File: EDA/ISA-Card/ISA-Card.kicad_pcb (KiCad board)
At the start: 2 copper layers, 138.4 x 98.4 mm, 161 parts, among them U7101 74HCT245, U7102 74HCT244, U7104 74HCT138, U7105 74HCT138, U7106 74LS08, U7107 74LS32, U7108 74LS32, U7109 74HC368, U7110 74HC04, U7111 74HC125, U7112 74HC74, U7113 74HC74, U7114 74HC4024, U7115 74HC4024, U7116 74HC595, U7117 74HC595, U7118 74HC595, U7119 8251, U7120 26LS31, U7121 26LS32, X2 Conn_02x04_Counter_Clockwise, X3 DB15_Female, X5 Conn_02x08_Counter_Clockwise

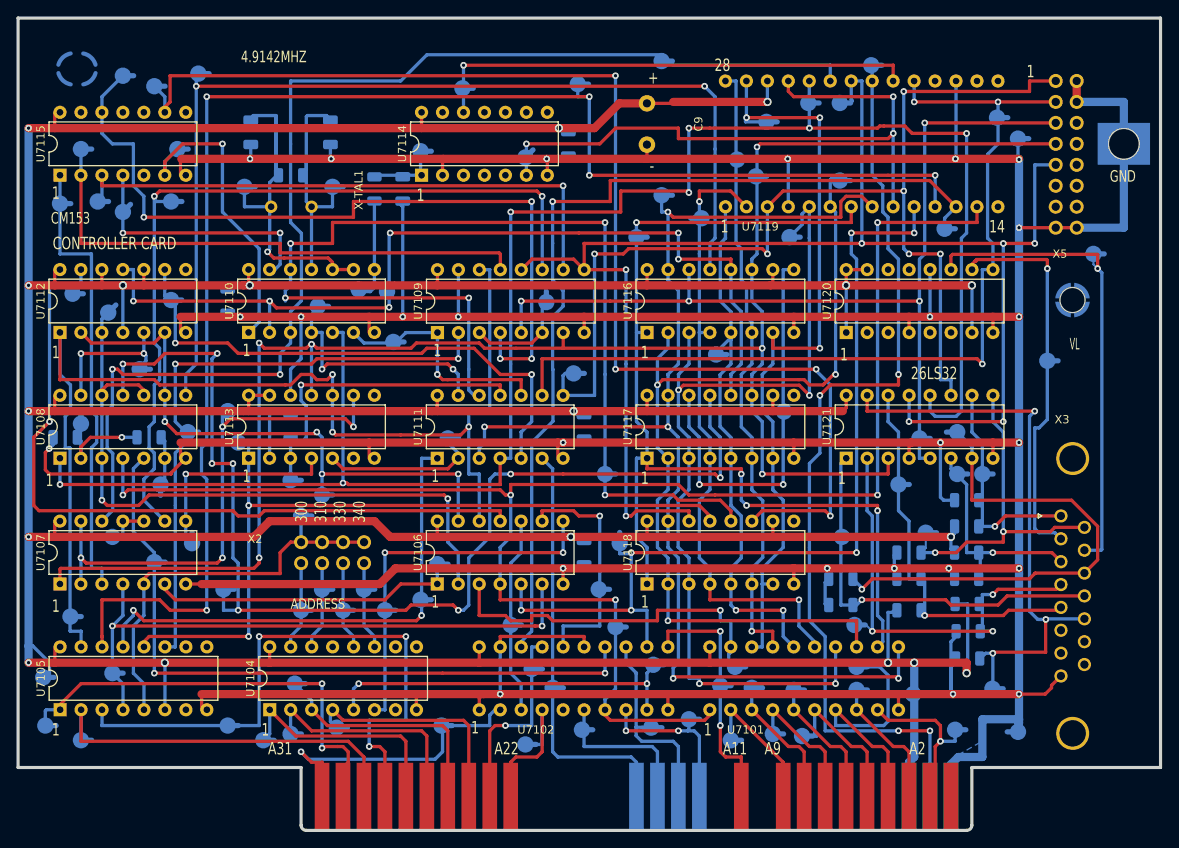
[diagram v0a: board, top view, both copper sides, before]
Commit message: Final cleanup complete
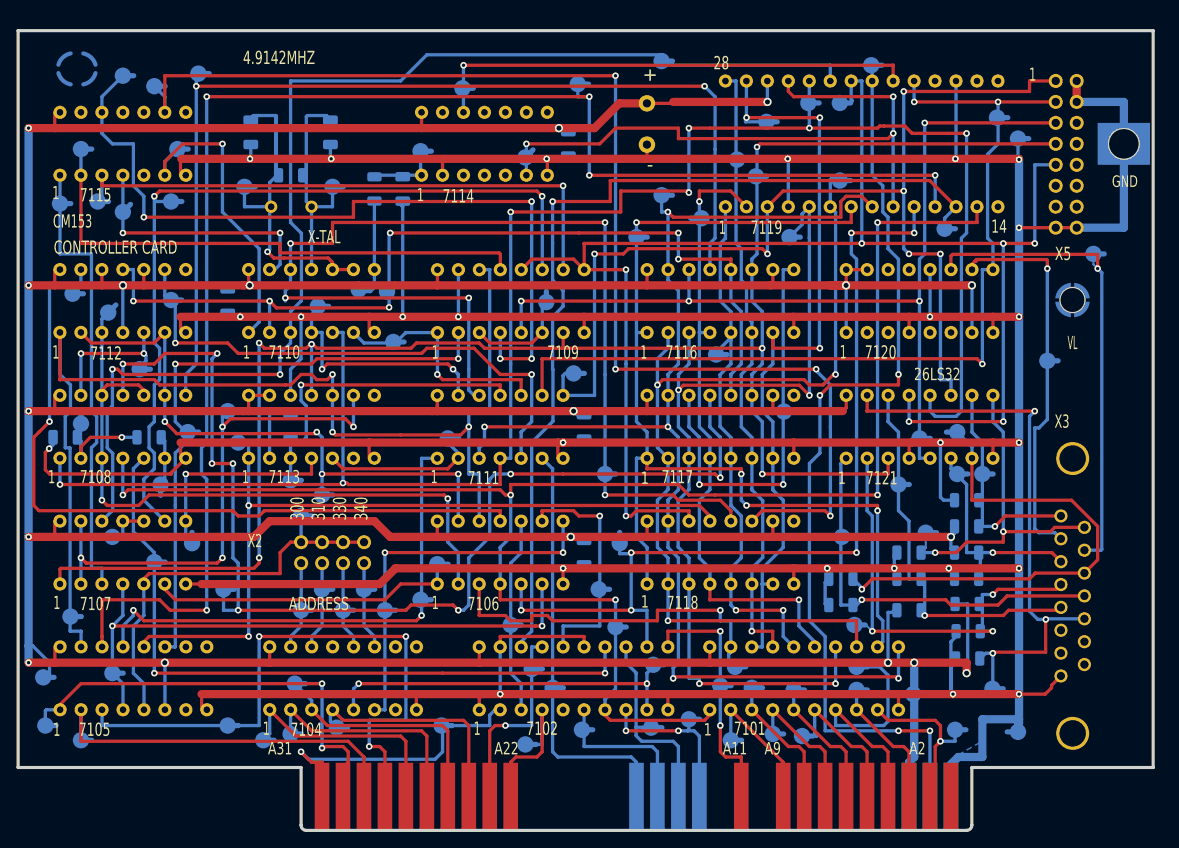
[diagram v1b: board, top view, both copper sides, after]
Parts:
- 7104: renamed from U7104; footprint Package_DIP:DIP-16_W7.62mm -> Philips-Shapes:DIP-16-Plain
- 7105: renamed from U7105; footprint Package_DIP:DIP-16_W7.62mm -> Philips-Shapes:DIP-16-Plain
- 7106: renamed from U7106; footprint Package_DIP:DIP-14_W7.62mm -> Philips-Shapes:DIP-14-Plain
- 7107: renamed from U7107; footprint Package_DIP:DIP-14_W7.62mm -> Philips-Shapes:DIP-14-Plain
- 7108: renamed from U7108; footprint Package_DIP:DIP-14_W7.62mm -> Philips-Shapes:DIP-14-Plain
- 7109: renamed from U7109; footprint Package_DIP:DIP-16_W7.62mm -> Philips-Shapes:DIP-16-Plain
- 7110: renamed from U7110; footprint Package_DIP:DIP-14_W7.62mm -> Philips-Shapes:DIP-14-Plain
- 7111: renamed from U7111; footprint Package_DIP:DIP-14_W7.62mm -> Philips-Shapes:DIP-14-Plain
- 7112: renamed from U7112; footprint Package_DIP:DIP-14_W7.62mm -> Philips-Shapes:DIP-14-Plain
- 7113: renamed from U7113; footprint Package_DIP:DIP-14_W7.62mm -> Philips-Shapes:DIP-14-Plain
- 7114: renamed from U7114; footprint Package_DIP:DIP-14_W7.62mm -> Philips-Shapes:DIP-14-Plain
- 7115: renamed from U7115; footprint Package_DIP:DIP-14_W7.62mm -> Philips-Shapes:DIP-14-Plain
- 7116: renamed from U7116; footprint Package_DIP:DIP-16_W7.62mm -> Philips-Shapes:DIP-16-Plain
- 7117: renamed from U7117; footprint Package_DIP:DIP-16_W7.62mm -> Philips-Shapes:DIP-16-Plain
- 7118: renamed from U7118; footprint Package_DIP:DIP-16_W7.62mm -> Philips-Shapes:DIP-16-Plain
- 7120: renamed from U7120; footprint Package_DIP:DIP-16_W7.62mm -> Philips-Shapes:DIP-16-Plain
- 7121: renamed from U7121; footprint Package_DIP:DIP-16_W7.62mm -> Philips-Shapes:DIP-16-Plain
- C1, C2, C3, C4, C5, C6, C7, C8: footprint Capacitor_SMD:C_1206_3216Metric -> Philips-Shapes:C_1206-Clean
- R1, R10, R11, R12, R13, R14, R15, R16, R2, R3, R4, R5, R6, R7, R8, R9: footprint Resistor_SMD:R_1206_3216Metric -> Philips-Shapes:R_1206-Clean
- renumbered U7101 to 7101, U7102 to 7102, U7119 to 7119, X-TAL1 to X-TAL
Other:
- board size 138.4 x 98.4 mm -> 137.5 x 96.9 mm
